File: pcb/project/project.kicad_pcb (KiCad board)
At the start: 2 copper layers, 28.5 x 65 mm, 3 parts, among them J1 110990030, J2 Conn_01x04_Pin, U1 DFR0654

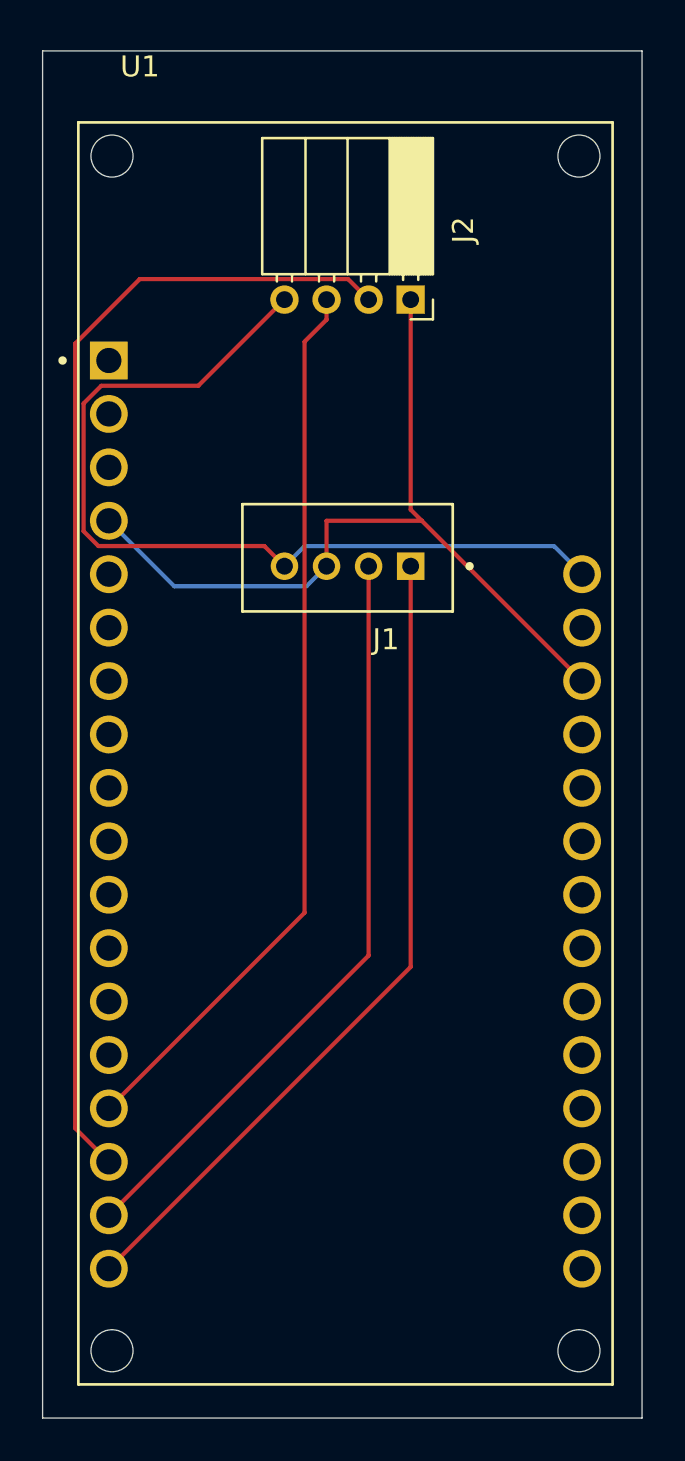
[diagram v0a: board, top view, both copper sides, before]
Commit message: PCB_2eversie
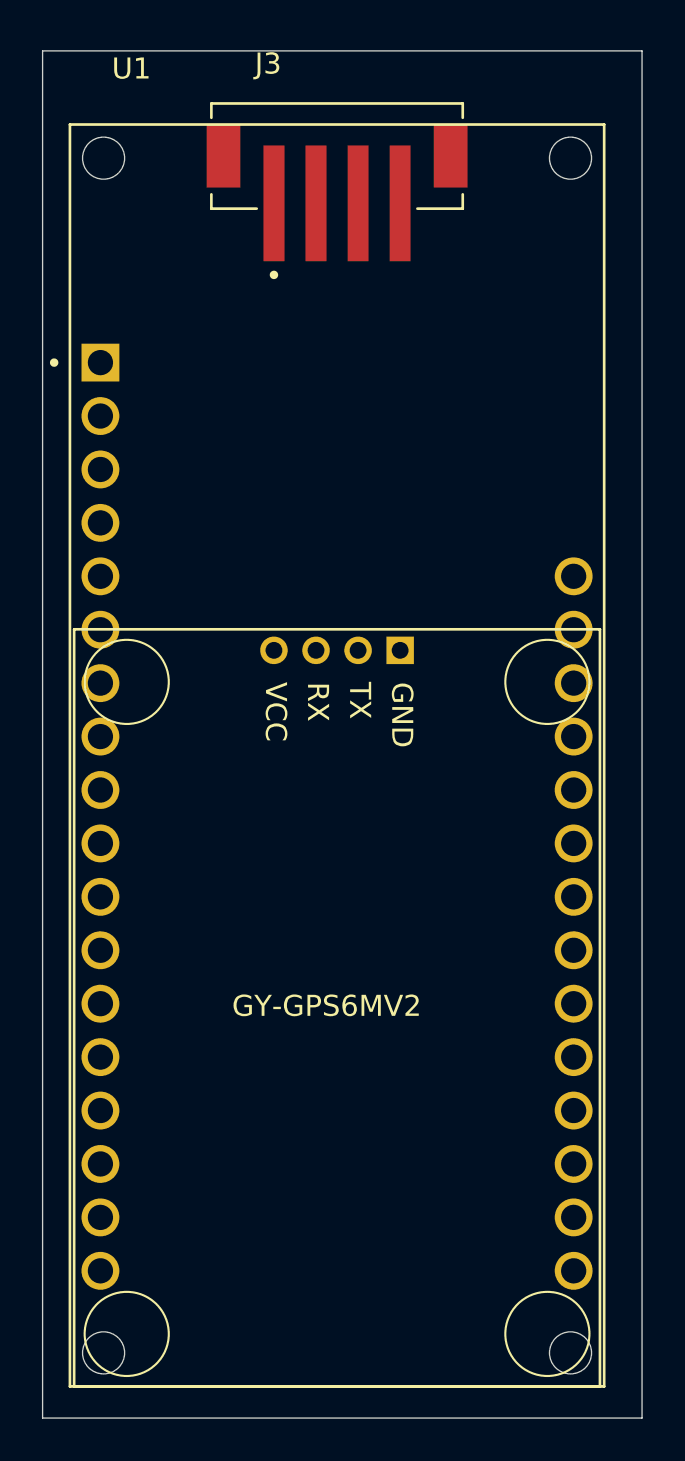
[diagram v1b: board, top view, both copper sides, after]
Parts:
- removed J2: Conn_01x04_Pin, Connector_PinSocket_2.00mm:PinSocket_1x04_P2.00mm_Horizontal
- added J3: B4B-PH-SM4-TB__LF__SN_, Footprints:JST_B4B-PH-SM4-TB__LF__SN_, F.Cu at (170.0, 63.5)
- J1: footprint warre:SEEED_110990030 -> Footprints:GY-GPS6MV2
- moved J1 21.0 mm to (170.0, 104.0), turned to 0 degrees
- moved U1 0.41 mm to (170.0, 92.0)
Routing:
- net TX: track 55.2 -> 0.00 mm
- net vcc: track 43.0 -> 0.00 mm
- net RX: track 42.7 -> 0.00 mm
- net GND: track 40.2 -> 0.00 mm
- net TX_1: track 39.3 -> 0.00 mm
- net RX_1: track 36.0 -> 0.00 mm
